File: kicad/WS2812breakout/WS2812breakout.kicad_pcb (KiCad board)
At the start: 2 copper layers, 5.4 x 9.9 mm, 3 parts, among them J3 Conn_01x04_Socket

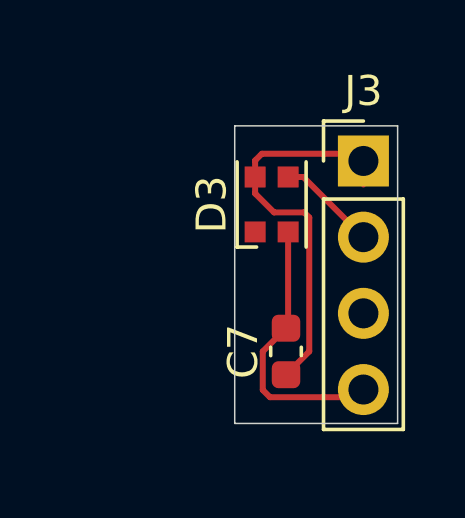
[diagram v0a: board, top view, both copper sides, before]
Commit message: Routed and Prettied-up breakout board
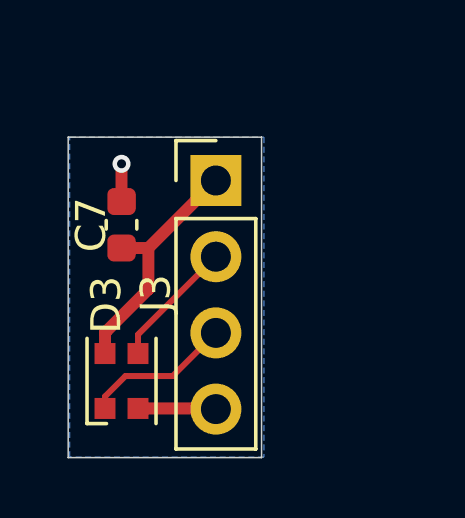
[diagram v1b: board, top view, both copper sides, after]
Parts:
- moved D3 7.72 mm to (116.3, 58.5)
- moved C7 6.92 mm to (116.3, 53.3)
- moved J3 4.96 mm to (119.5, 51.9)
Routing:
- net GND: track 9.18 -> 3.86 mm, vias 0 -> 1
- net +5V: track 13.4 -> 8.19 mm
- net /OUT: track 0.00 -> 4.97 mm
- net /IN: track 3.34 -> 4.30 mm
- added copper zone on B.Cu, net GND
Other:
- board size 5.4 x 9.9 mm -> 6.4 x 10.7 mm
- board text added: "AG/CJ"
- board text added: "Breakout v1"
- board text added: "WS2812b"
